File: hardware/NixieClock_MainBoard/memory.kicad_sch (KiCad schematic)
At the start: 3 parts, among them J7 Micro_SD_Card

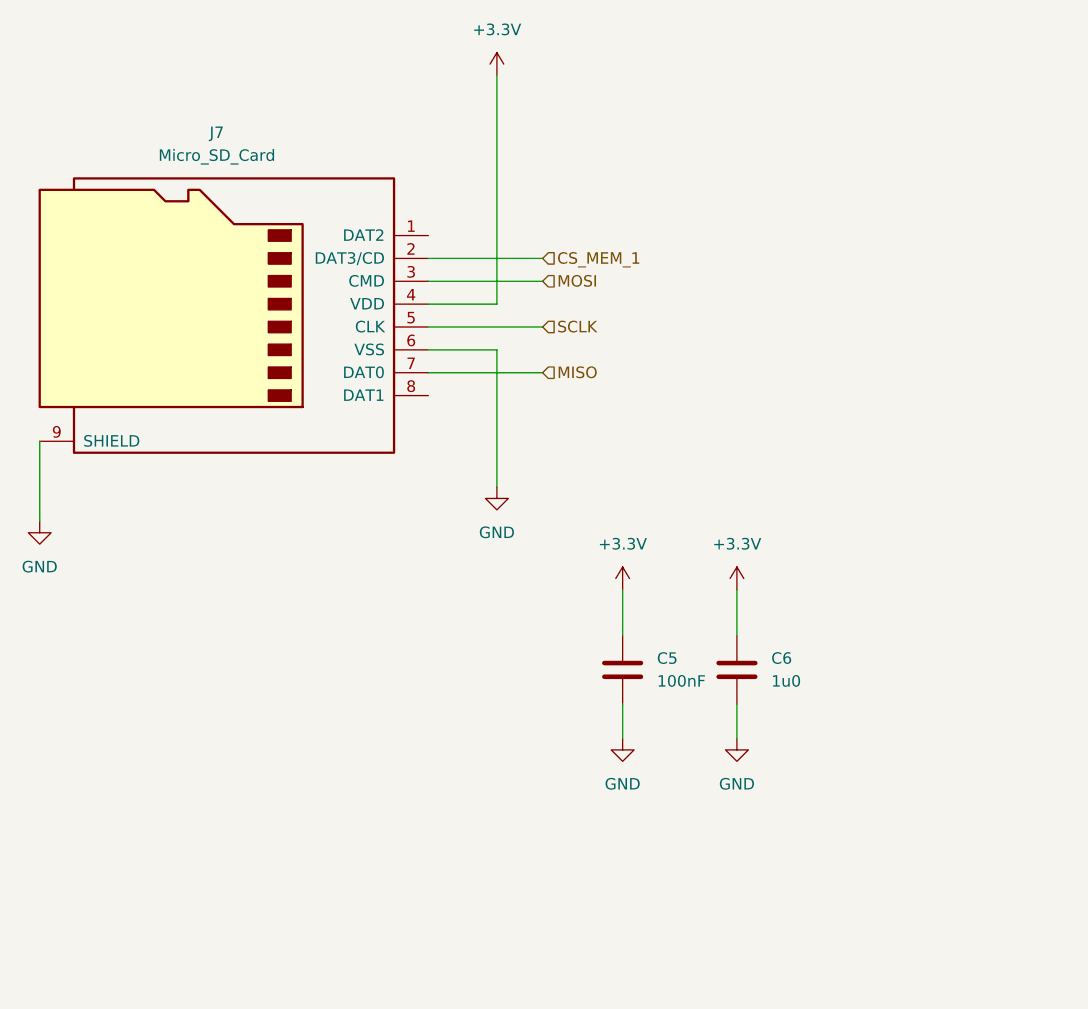
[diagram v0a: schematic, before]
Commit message: V2.0 release fertig.
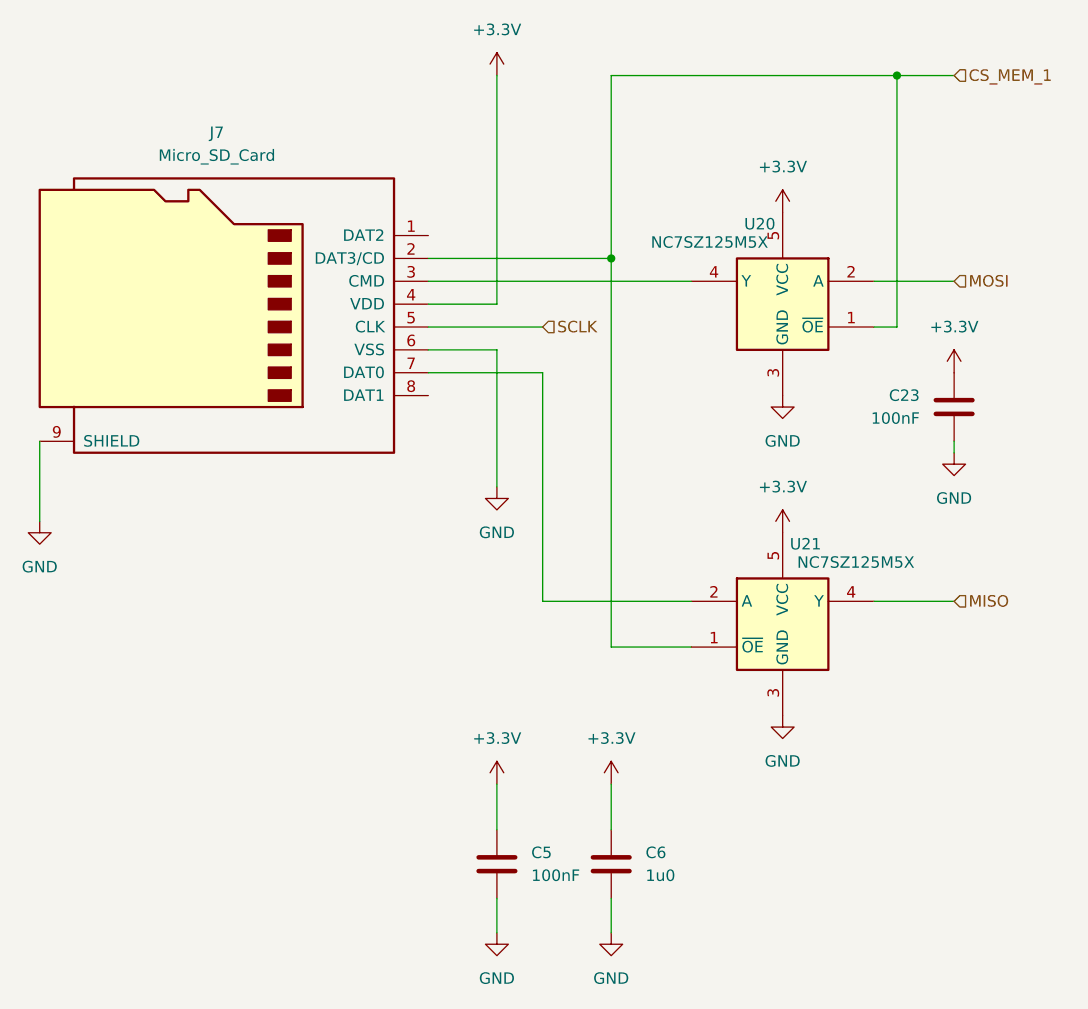
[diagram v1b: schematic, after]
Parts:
- added C23: 100nF, Capacitor_SMD:C_0603_1608Metric, symbol Device:C
- added U20, U21: NC7SZ125M5X, Package_TO_SOT_SMD:SOT-23-5, symbol 74xGxx:NC7SZ125M5X
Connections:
- net +3.3V: now also C23.1, U20.5 (VCC), U21.5 (VCC)
- net CS_MEM_1: now also U20.1 (~{OE}), U21.1 (~{OE})
- net GND: now also C23.2, U20.3 (GND), U21.3 (GND)
- net MISO: now also U21.4 (Y); no longer J7.7 (DAT0)
- net MOSI: now also U20.2 (A); no longer J7.3 (CMD)
- new net: J7.3 (CMD), U20.4 (Y)
- new net: J7.7 (DAT0), U21.2 (A)
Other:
- moved on the sheet: C5, C6
